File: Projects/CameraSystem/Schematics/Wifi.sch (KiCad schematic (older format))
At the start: 4 parts, among them U4 ESP8266

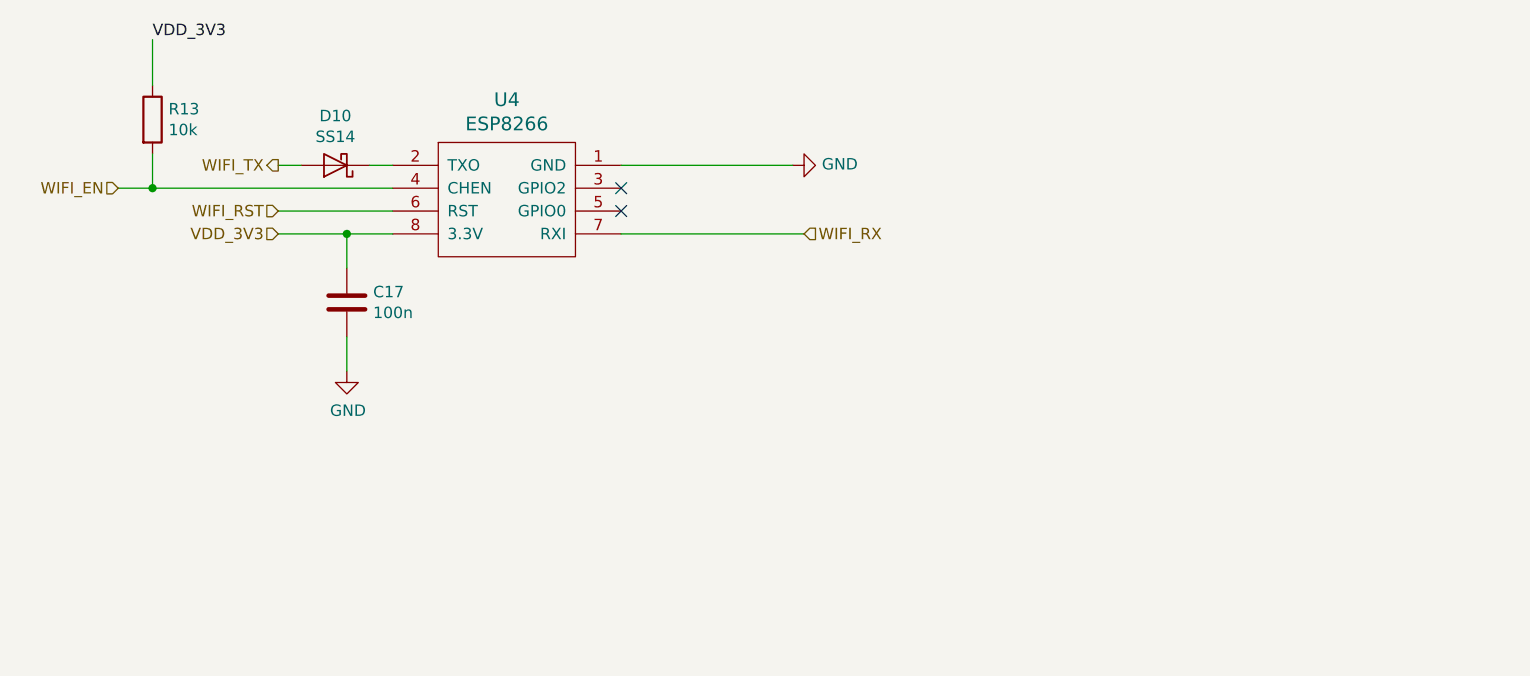
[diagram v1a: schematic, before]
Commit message: nothing hcanged
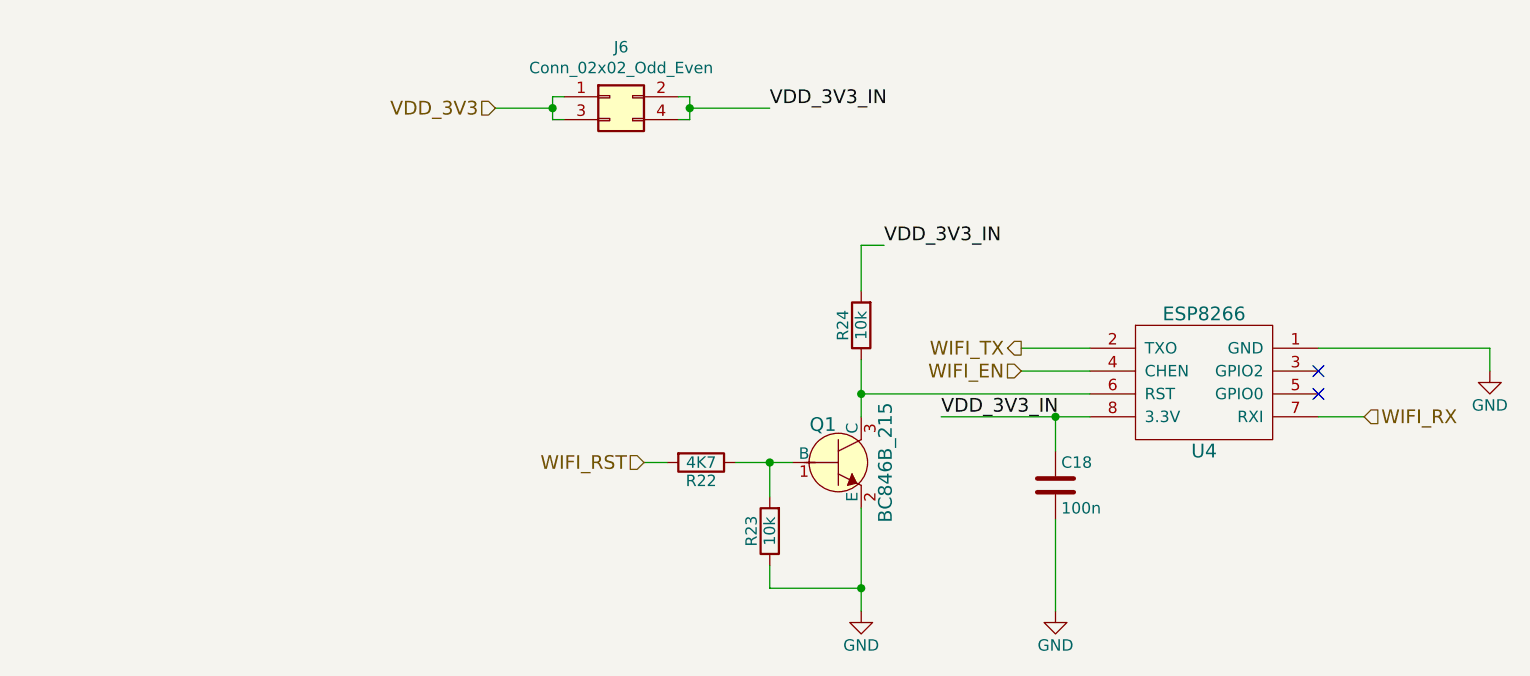
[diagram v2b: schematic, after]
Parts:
- removed C17: 100n, Capacitor_SMD:C_0603_1608Metric_Pad1.05x0.95mm_HandSolder, symbol Device:C
- removed D10: SS14, custom-footprints:SMA_DO-214AC, symbol Device:D_Schottky
- removed R13: 10k, Resistor_SMD:R_0603_1608Metric_Pad1.05x0.95mm_HandSolder, symbol Device:R
- added C18: 100n, digikey-footprints:0603, symbol Device:C
- added J6: Conn_02x02_Odd_Even, Pin_Headers:Pin_Header_Straight_2x02_Pitch2.54mm_SMD, symbol Connector_Generic:Conn_02x02_Odd_Even
- added Q1: BC846B_215, digikey-footprints:SOT-23-3, symbol CameraSystem-rescue:BC846B_215
- added R22: 4K7, digikey-footprints:0603, symbol Device:R
- added R23, R24: 10k, digikey-footprints:0603, symbol Device:R
- U4: footprint Connector_PinSocket_2.54mm:PinSocket_2x04_P2.54mm_Vertical -> Pin_Headers:Pin_Header_Straight_2x04_Pitch2.54mm
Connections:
- net GND: now also C18.2, Q1.2 (E), R23.1
- net VDD_3V3: now also J6.1 (Pin_1), J6.3 (Pin_3); no longer U4.8 (3.3V)
- net WIFI_RST: now also R22.2; no longer U4.6 (RST)
- net WIFI_TX: now also U4.2 (TXO)
- new net: Q1.3 (C), R24.1, U4.6 (RST)
- new net: Q1.1 (B), R22.1, R23.2
- new net VDD_3V3_IN: C18.1, J6.2 (Pin_2), J6.4 (Pin_4), R24.2, U4.8 (3.3V)
